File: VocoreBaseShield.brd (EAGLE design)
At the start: 25.7 x 25.7 mm, 7 parts, among them U1 VOCORE_SHIELD

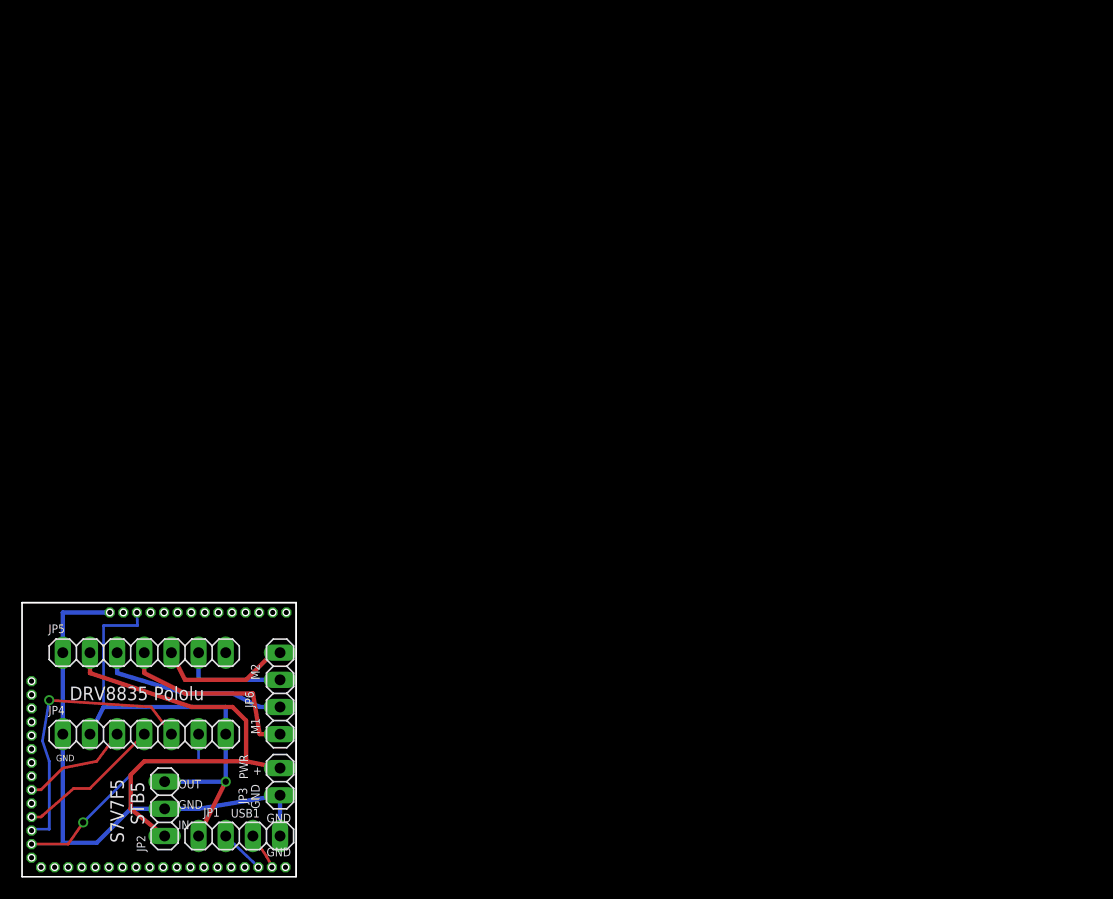
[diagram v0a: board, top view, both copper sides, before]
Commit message: Revert "Version 0.1"
This reverts commit b4409390f012a34cf1db7157863f4cbc9e08abe1.
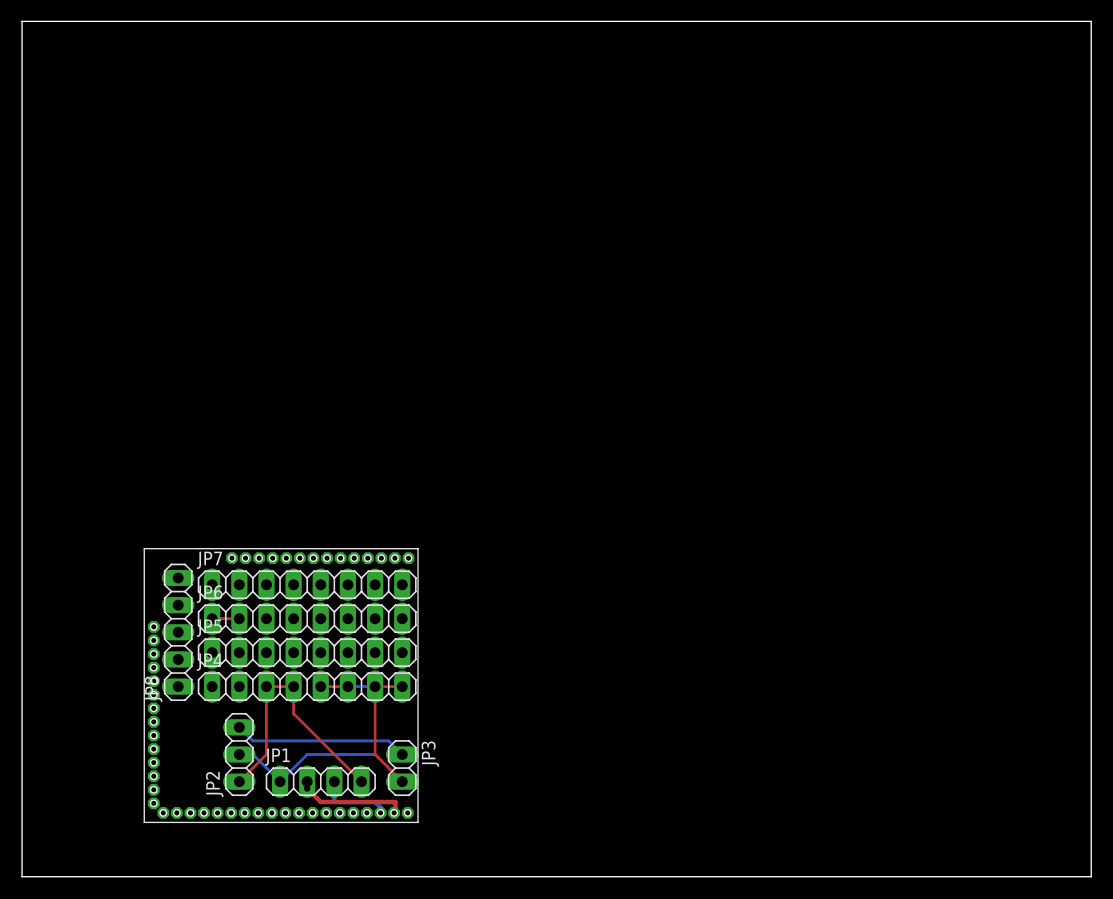
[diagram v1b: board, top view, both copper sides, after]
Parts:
- removed U1: VOCORE_SHIELD, Vocore:VOCORE_DOC_CUSTOM
- added JP7: (no value), pinhead:1X08
- added JP8: (no value), pinhead:1X05
- added U$1: VOCORE_SHIELD, Vocore:VOCORE_DOC_CUSTOM
- JP4, JP5: device pinhead:1X07 -> pinhead:1X08
- JP6: device pinhead:1X04 -> pinhead:1X08
- moved JP4 15.9 mm to (26.7, 17.8)
- moved JP5 15.2 mm to (26.7, 21.0)
- moved JP3 11.5 mm to (35.6, 10.2)
- moved JP1 9.16 mm to (27.9, 8.89), turned to 0 degrees
- moved JP2 8.64 mm to (20.3, 11.4), turned to 90 degrees
- moved JP6 7.43 mm to (26.7, 24.1), turned to 0 degrees
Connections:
- new net N$12: JP5.5, U$1.G#24/LED2
- new net N$15: JP5.8, U$1.G#27/SPI_CS1
- new net N$16: JP6.8, U$1.G#14/PCM_TDX
- new net N$17: JP6.7, U$1.G#13/PCM_DRX
- new net N$18: JP6.6, U$1.G#12/PCM_CLK
- new net N$19: JP6.5, U$1.G#11/PCM_FS
- new net N$20: JP6.4, U$1.G#10/I2S_SDI/RXD
- new net N$21: JP6.3, U$1.G#09/I2S_SDO
- new net N$22: JP6.1, JP6.2, U$1.G#08/I2S_WS/TXD
- new net N$23: JP7.1, U$1.RESET
- new net N$24: JP7.2, U$1.G#00
- new net N$25: JP7.3, U$1.G#01/I2C_CLK
- new net N$26: JP7.4, U$1.G#02/I2C_SD
- new net N$27: JP7.5, U$1.G#03/SPI_CS0
- new net N$28: JP7.6, U$1.G#04/SPI_CLK
- new net N$29: JP7.7, U$1.G#05/SPI_MOSI
- new net N$30: JP7.8, U$1.G#06/SPI_MISO
- new net N$31: JP8.2, U$1.G#20/JTAG_TCLK
- new net N$32: U$1.G#19/JTAG_TMS
- new net N$33: JP8.4, U$1.G#18/JTAG_TDI
- new net N$34: JP8.1, U$1.G#21/JTAG_TRST
- new net N$35: JP8.5, U$1.G#17/JTAG_TDO
- net N$1: now also JP4.5, JP4.6, JP4.7, JP4.8, U$1.GND, U$1.GND1, U$1.GND2, U$1.GND3; no longer JP4.1, JP5.1, U1.GND2
- net N$10: now also JP5.3, U$1.G#22/LED0; no longer JP5.4, JP6.1
- net N$11: now also JP5.4, U$1.G#23/LED1; no longer JP5.3, JP6.2
- net N$13: now also JP5.6, U$1.G#25/LED3; no longer JP5.5, JP6.4
- net N$14: now also JP5.7, U$1.G#26/LED4; no longer JP5.6, JP6.3
- net N$2: no longer JP5.2
- net N$3: now also JP4.3, JP4.4, U$1.+6.0VIN, U$1.+6.0VIN1; no longer JP4.2, JP4.7, U1.+6.0VIN1
- net N$4: now also JP4.1, U$1.+1.8V; no longer JP4.3, U1.G#23/LED1
- net N$5: now also U$1.USB-; no longer U1.USB-
- net N$6: now also U$1.USB+; no longer U1.USB+
- net N$7: now also JP4.2, U$1.+3.2V~+3.5V; no longer JP4.4, U1.G#24/LED2
- net N$8: now also JP5.1, U$1.G#15/TXD2; no longer JP4.5, U1.G#25/LED3
- net N$9: now also JP5.2, U$1.G#16/RXD2; no longer JP4.6, U1.G#26/LED4
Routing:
- net N$2: track 43.2 -> 16.3 mm
- net N$8: track 26.6 -> 0.00 mm, vias 1 -> 0
- net N$9: track 21.6 -> 0.00 mm, vias 1 -> 0
- net N$3: track 44.7 -> 24.0 mm, vias 1 -> 0
- net N$10: track 18.3 -> 0.00 mm
- net N$11: track 17.7 -> 0.00 mm
- net N$1: track 51.5 -> 36.0 mm, vias 1 -> 0
- net N$7: track 13.6 -> 0.00 mm
- net N$13: track 12.8 -> 0.00 mm
- net N$4: track 10.2 -> 0.00 mm
- net N$14: track 10.2 -> 0.00 mm
- net N$6: track 3.78 -> 10.5 mm, vias 0 -> 1
- net N$5: track 4.22 -> 6.94 mm
- net N$22: track 0.00 -> 2.54 mm
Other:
- board size 25.7 x 25.7 mm -> 100 x 80 mm
- board text removed: "+"
- board text removed: "DRV8835 Pololu"
- board text removed: "GND"
- board text removed: "IN"
- board text removed: "M1"
- board text removed: "M2"
- board text removed: "OUT"
- board text removed: "S7V7F5"
